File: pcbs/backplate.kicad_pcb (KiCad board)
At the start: 2 copper layers, 114 x 91.6 mm, 5 parts

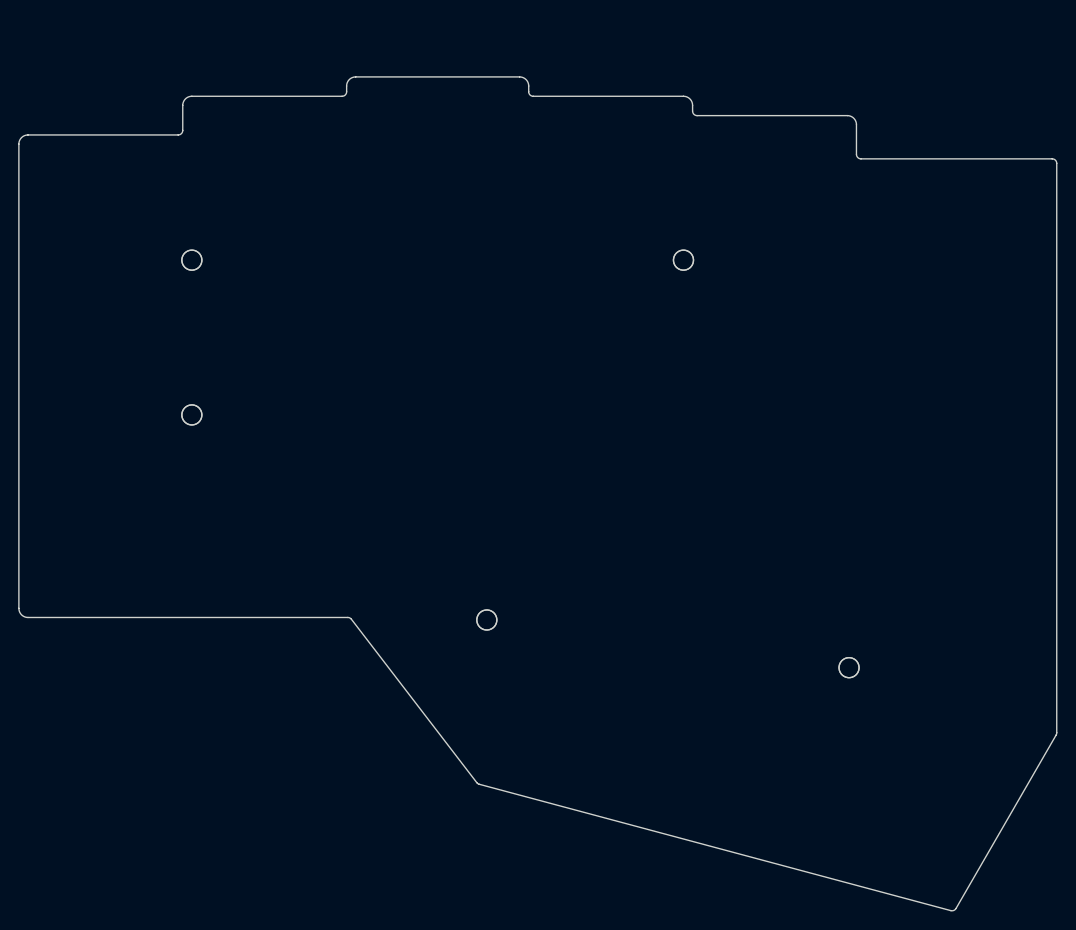
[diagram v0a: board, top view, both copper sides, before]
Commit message: staggero_change
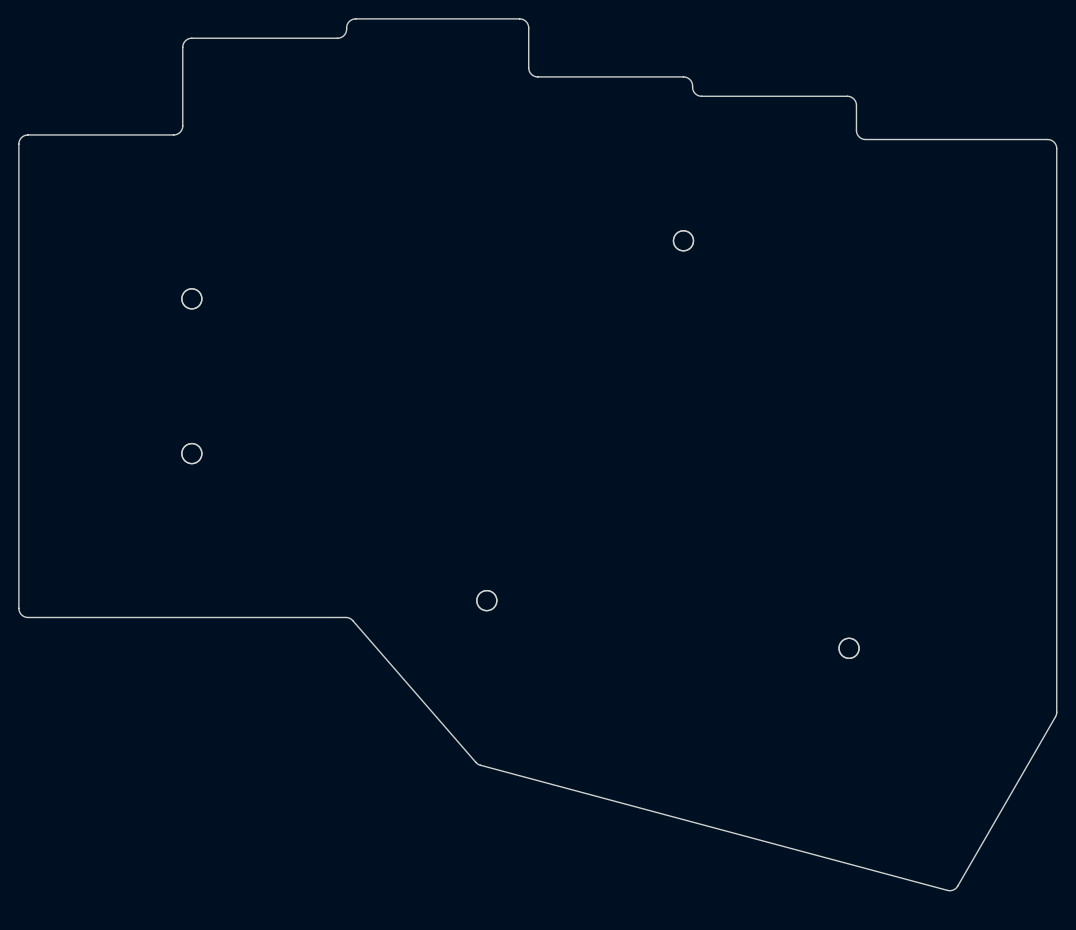
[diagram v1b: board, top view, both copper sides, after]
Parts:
- moved MH1 4.25 mm to (109.0, 74.5)
- moved MH2 4.25 mm to (109.0, 91.5)
- moved MH3 2.12 mm to (163.0, 68.1)
- moved MH4 2.12 mm to (141.4, 107.7)
- moved MH5 2.12 mm to (181.2, 112.9)
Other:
- board size 114 x 91.6 mm -> 114 x 95.8 mm
